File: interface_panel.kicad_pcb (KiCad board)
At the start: 2 copper layers, 69.3 x 32.4 mm, 13 parts, among them J1 Conn_02x04_Odd_Even

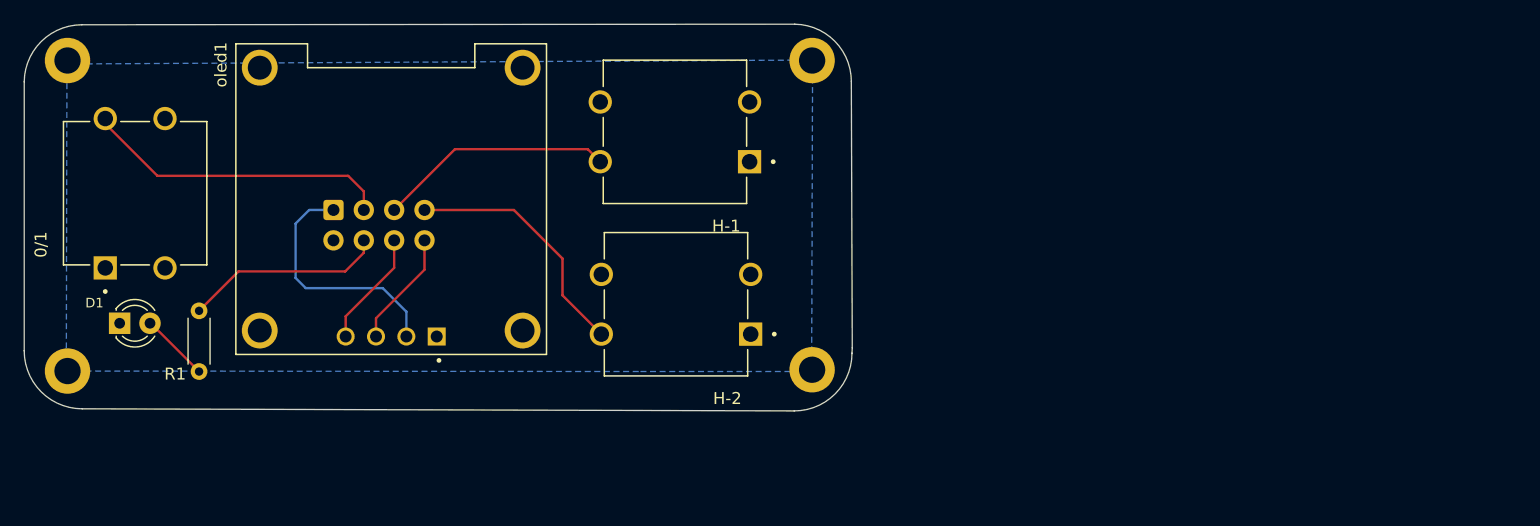
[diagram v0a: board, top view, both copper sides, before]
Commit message: production level changes -1
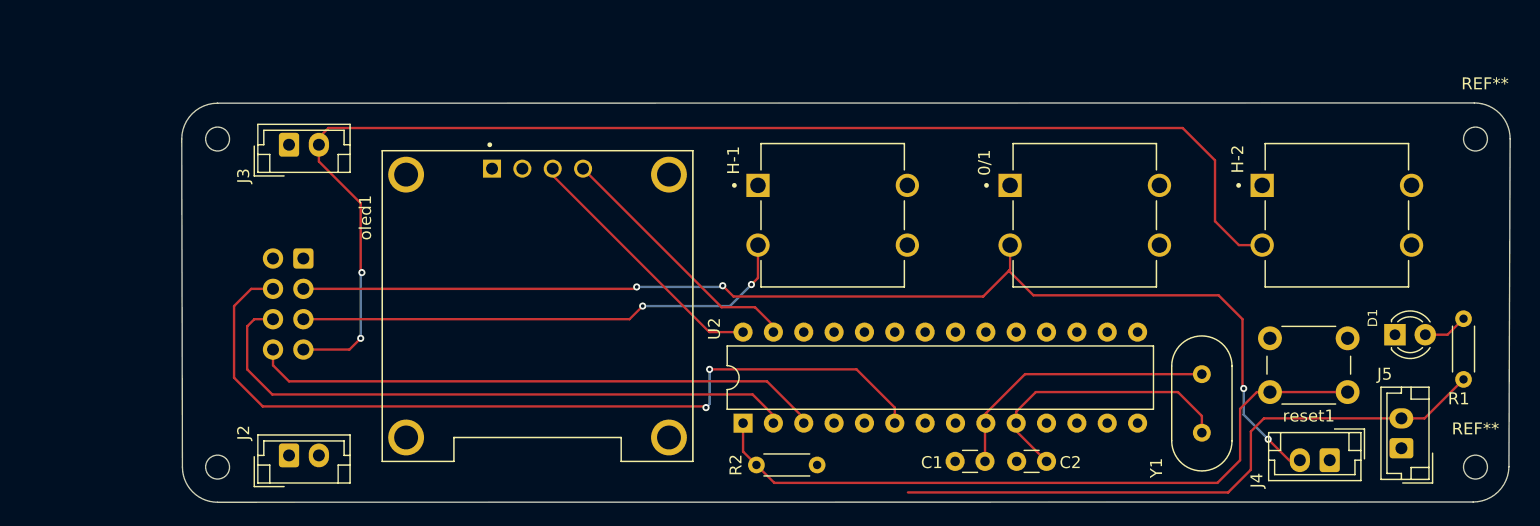
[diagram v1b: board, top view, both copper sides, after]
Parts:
- removed the REF** at (178.3, 63.5)
- removed the REF** at (116.0, 63.5)
- removed the REF** at (178.3, 89.4)
- removed the REF** at (151.6, 62.5)
- removed the REF** at (116.0, 89.5)
- removed the REF** at (161.1, 63.2)
- added C1: C, Capacitor_THT:C_Disc_D3.0mm_W1.6mm_P2.50mm, F.Cu at (192.8, 97.1)
- added C2: C, Capacitor_THT:C_Disc_D3.0mm_W1.6mm_P2.50mm, F.Cu at (197.9, 97.1)
- added J2: but1, Connector_JST:JST_EH_B2B-EH-A_1x02_P2.50mm_Vertical, F.Cu at (134.5, 96.6)
- added J3: but2, Connector_JST:JST_EH_B2B-EH-A_1x02_P2.50mm_Vertical, F.Cu at (134.5, 70.6)
- added J4: but3, Connector_JST:JST_EH_B2B-EH-A_1x02_P2.50mm_Vertical, F.Cu at (221.6, 97.0)
- added J5: Led, Connector_JST:JST_EH_B2B-EH-A_1x02_P2.50mm_Vertical, F.Cu at (227.6, 96.0)
- added R2: 10k, Resistor_THT:R_Axial_DIN0204_L3.6mm_D1.6mm_P5.08mm_Horizontal, F.Cu at (173.6, 97.4)
- added REF**: MountingHole_2mm, MountingHole:MountingHole_2mm, F.Cu at (233.8, 97.6)
- added REF**: MountingHole_2mm, MountingHole:MountingHole_2mm, F.Cu at (128.5, 97.6)
- added REF**: MountingHole_2mm, MountingHole:MountingHole_2mm, F.Cu at (233.8, 70.1)
- added REF**: MountingHole_2mm, MountingHole:MountingHole_2mm, F.Cu at (128.5, 70.1)
- added U2: ATmega328P-P, Package_DIP:DIP-28_W7.62mm, F.Cu at (172.5, 93.9)
- added Y1: Crystal, Crystal:Crystal_HC18-U_Vertical, F.Cu at (210.9, 94.7)
- added reset1: reset, Button_Switch_THT:SW_PUSH_6mm, F.Cu at (223.1, 91.3)
- moved D1 106.7 mm to (227.1, 86.5)
- moved R1 105.9 mm to (232.8, 85.2), turned to -90 degrees
- moved 0/1 79.5 mm to (201.1, 76.5), turned to 0 degrees
- moved H-2 55.8 mm to (222.2, 76.5), turned to 0 degrees
- moved oled1 15.2 mm to (155.3, 84.1), turned to 0 degrees
- moved H-1 14.9 mm to (180.0, 76.5), turned to 0 degrees
- moved J1 4.78 mm to (135.7, 80.1), turned to 180 degrees
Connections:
- J1 pad 6: SDA -> RX
- J1 pad 8: SCL -> TX
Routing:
- net S. LED: track 16.8 -> 124.1 mm, vias 0 -> 2
- net BT-2: track 20.9 -> 109.9 mm, vias 0 -> 2
- net BT-Pwr: track 26.0 -> 98.3 mm, vias 0 -> 4
- net Net-(U2-~{RESET}/PC6): track 0.00 -> 59.7 mm
- net RX: track 0.00 -> 52.3 mm
- net TX: track 0.00 -> 48.0 mm
- net Net-(U2-XTAL2/PB7): track 0.00 -> 23.7 mm
- net Net-(U2-XTAL1/PB6): track 0.00 -> 23.5 mm
- net BT-1: track 19.8 -> 42.2 mm, vias 0 -> 2
- net 5V: track 20.7 -> 0.00 mm
- net SCL: track 9.73 -> 21.9 mm
- net SDA: track 9.73 -> 21.9 mm
- net Net-(D1-A): track 0.00 -> 3.76 mm
- removed copper zone on B.Cu, net GND
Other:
- board size 69.3 x 32.4 mm -> 111.2 x 33.4 mm
